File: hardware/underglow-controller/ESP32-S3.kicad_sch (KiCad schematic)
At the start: 38 parts, among them J101 CONSOLE, SW101 SW_Push, SW102 SW_Push, U101 ESP32-S3R2, U102 W25Q128JVS, Y101 40MHZ

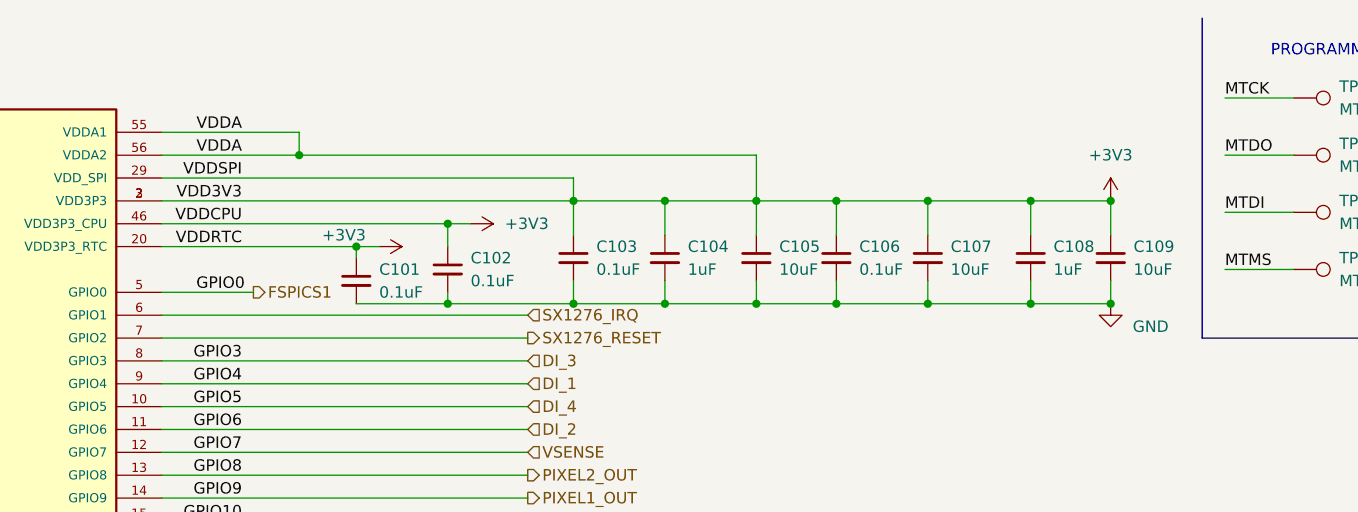
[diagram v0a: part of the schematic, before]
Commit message: Hardware updates, firmware updates blah blah blah
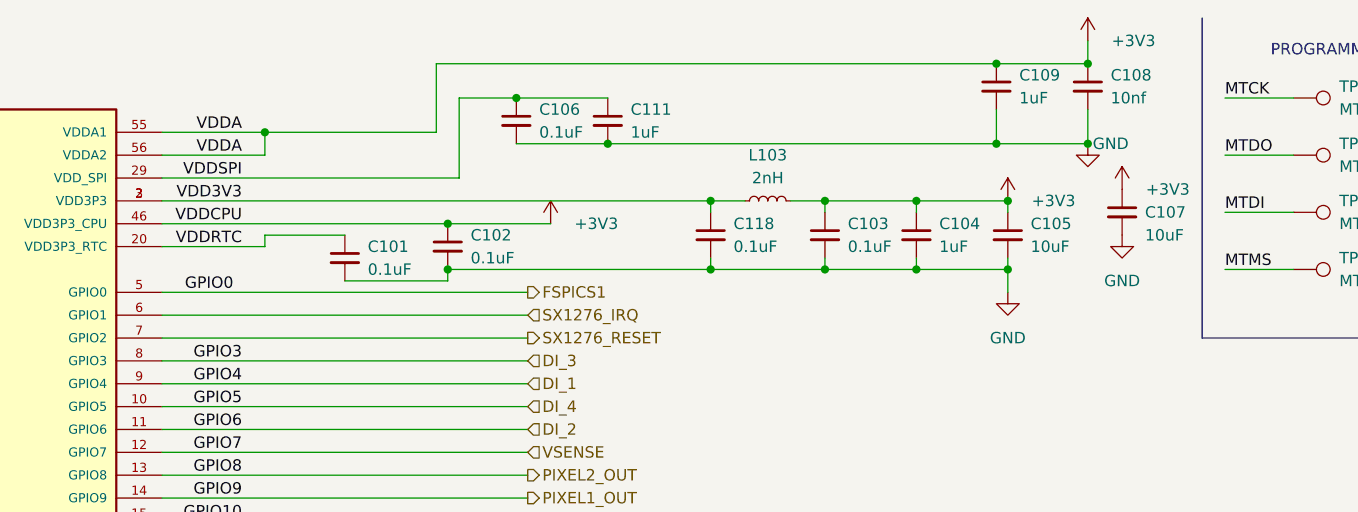
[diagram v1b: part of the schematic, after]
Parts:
- added C111: 1uF, Capacitor_SMD:C_0402_1005Metric, symbol Device:C_Small
- added C118: 0.1uF, Capacitor_SMD:C_0402_1005Metric, symbol Device:C_Small
- added L103: 2nH, Inductor_SMD:L_0402_1005Metric, symbol Device:L_Small
- C108: value 1uF -> 10nf; MPN CGA2B1X7T0G105M050BC -> (none)
- C109: value 10uF -> 1uF; MPN GRT21BC81A106KE01L -> (none)
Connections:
- net +3V3: now also L103.2; no longer C101.1, C106.1, C110.1, R105.1, U101.2 (VDD3P3), U101.20 (VDD3P3_RTC), U101.29 (VDD_SPI), U101.3 (VDD3P3), U102.8 (VCC)
- net GND: now also C111.2, C118.2
- new net VDD3V3: C118.1, L103.1, U101.2 (VDD3P3), U101.3 (VDD3P3)
- new net VDDRTC: C101.1, U101.20 (VDD3P3_RTC)
- new net VDDSPI: C106.1, C110.1, C111.1, R105.1, U101.29 (VDD_SPI), U102.8 (VCC)
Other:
- moved on the sheet: C101, C102, C103, C104, C105, C106, C107, C108, C109
